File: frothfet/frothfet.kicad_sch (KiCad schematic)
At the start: 8 parts, among them U1 ESP32-S3-DEVKITC

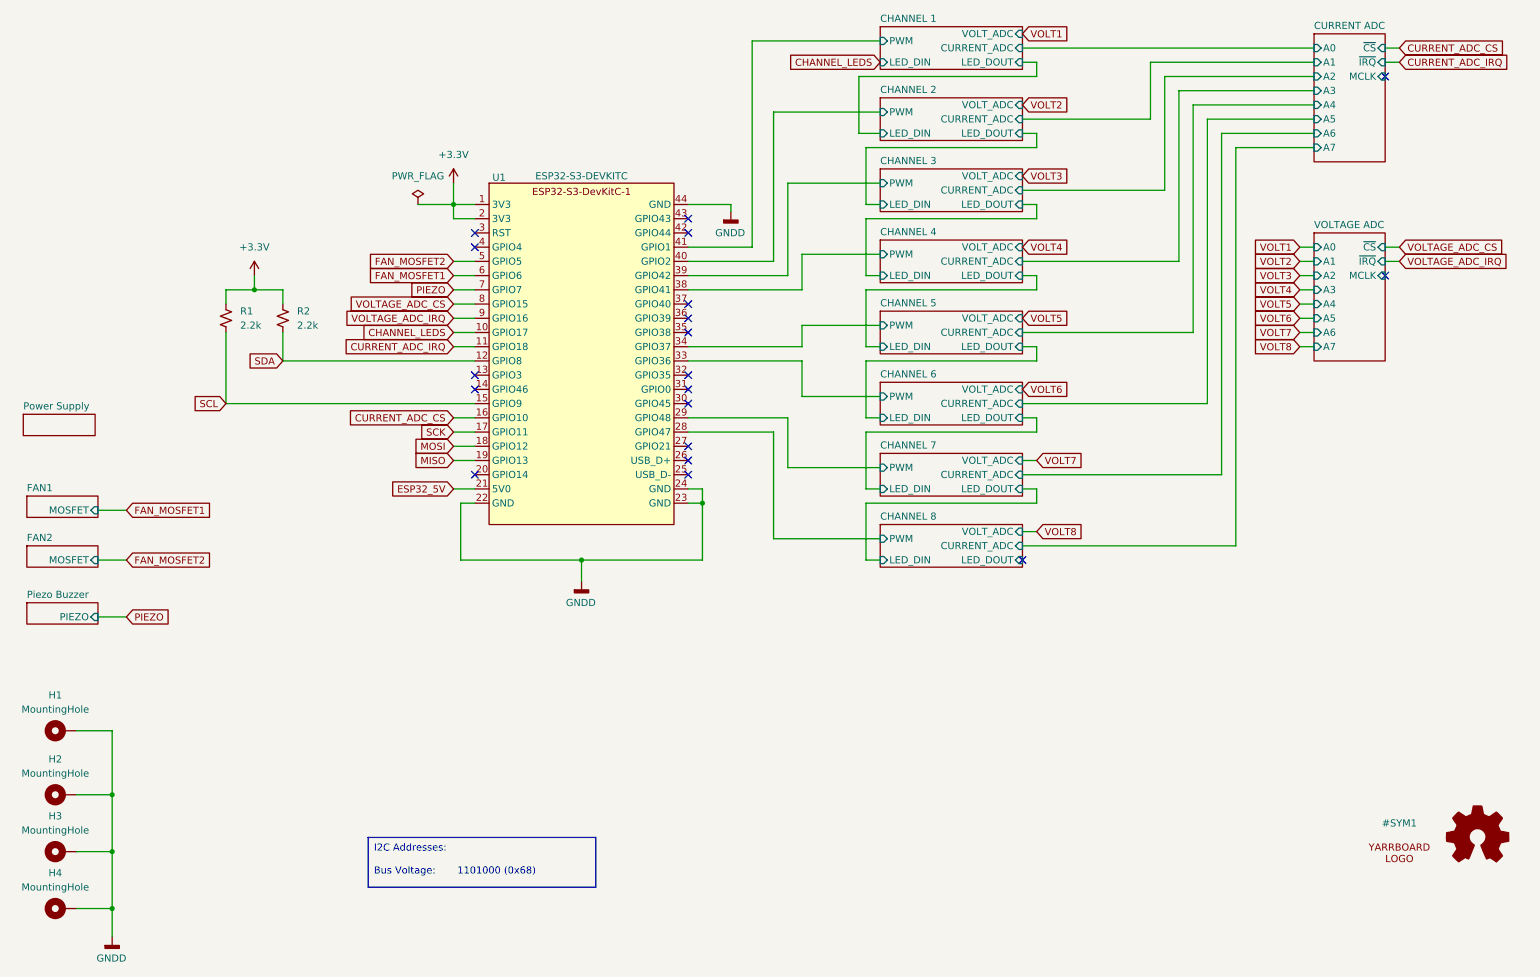
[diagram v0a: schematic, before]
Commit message: started work on rev e, looking clean at 13mm
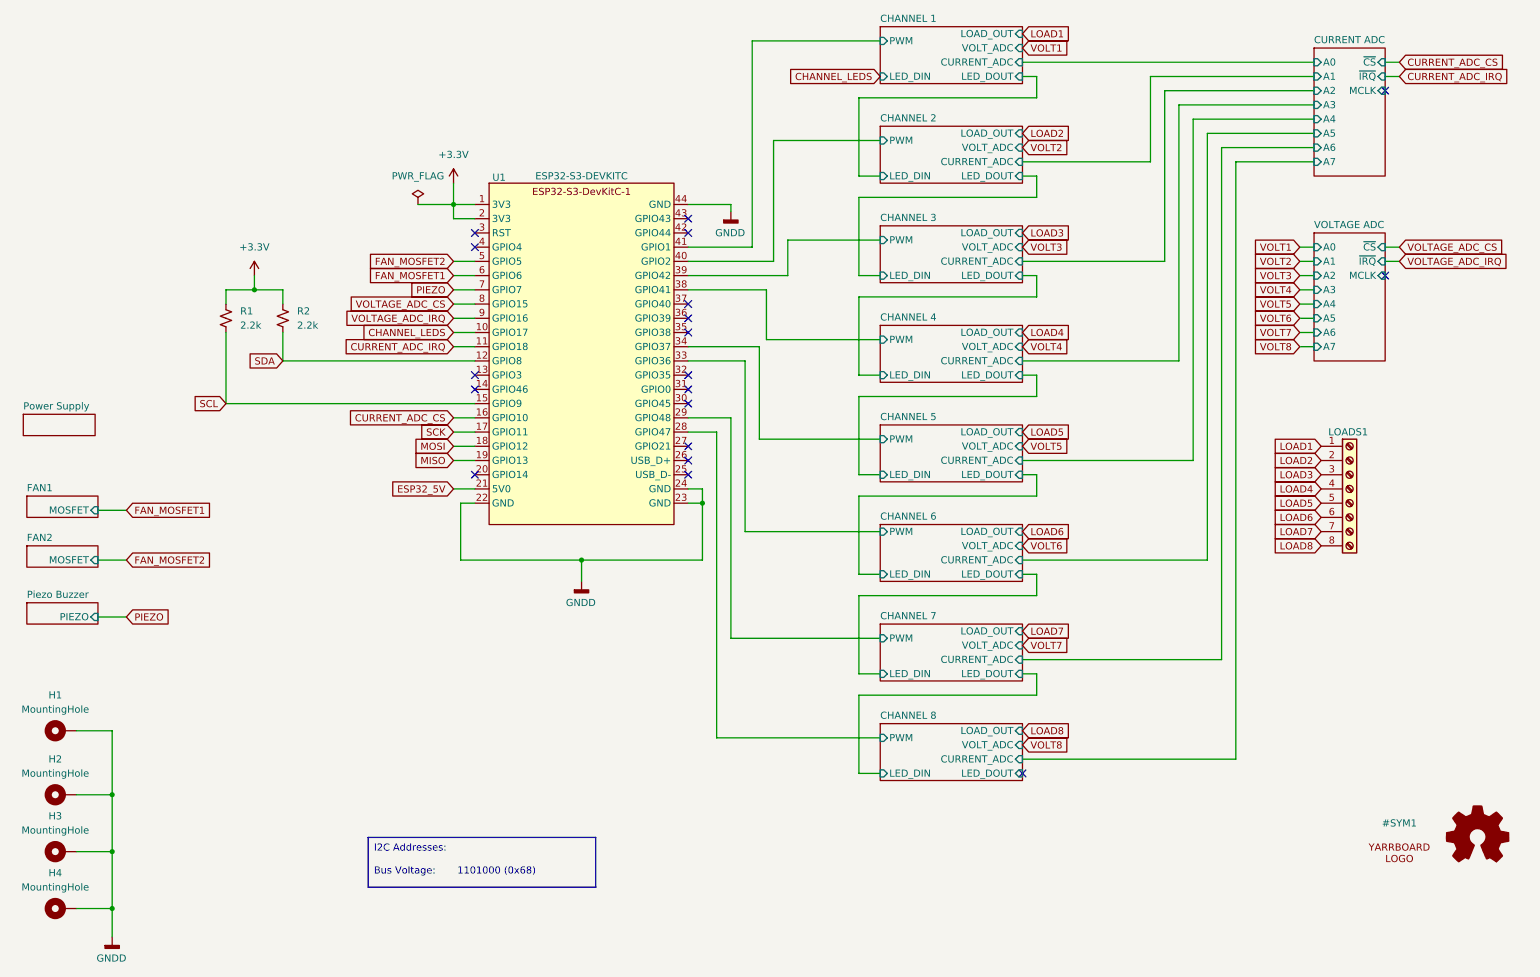
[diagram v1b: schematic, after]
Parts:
- added LOADS1: Screw_Terminal_01x08, yarrboard:KF78S-13.0-8P, symbol Connector:Screw_Terminal_01x08
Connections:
- new net LOAD1: LOADS1.1 (Pin_1)
- new net LOAD2: LOADS1.2 (Pin_2)
- new net LOAD3: LOADS1.3 (Pin_3)
- new net LOAD4: LOADS1.4 (Pin_4)
- new net LOAD5: LOADS1.5 (Pin_5)
- new net LOAD6: LOADS1.6 (Pin_6)
- new net LOAD7: LOADS1.7 (Pin_7)
- new net LOAD8: LOADS1.8 (Pin_8)
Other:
- sheet CHANNEL 1 ports: added LOAD_OUT; removed none
- sheet CHANNEL 2 ports: added LOAD_OUT; removed none
- sheet CHANNEL 3 ports: added LOAD_OUT; removed none
- sheet CHANNEL 4 ports: added LOAD_OUT; removed none
- sheet CHANNEL 5 ports: added LOAD_OUT; removed none
- sheet CHANNEL 6 ports: added LOAD_OUT; removed none
- sheet CHANNEL 7 ports: added LOAD_OUT; removed none
- sheet CHANNEL 8 ports: added LOAD_OUT; removed none
